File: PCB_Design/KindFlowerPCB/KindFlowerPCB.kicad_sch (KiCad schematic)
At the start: 13 parts, among them J1 LiPo_Connector, J2 FSR_1, J3 Wireless_Charger, J4 FSR_2, J5 FSR_3, J6 FSR_0, J7 NeopixelStrip1, J8 NeopixelStrip2

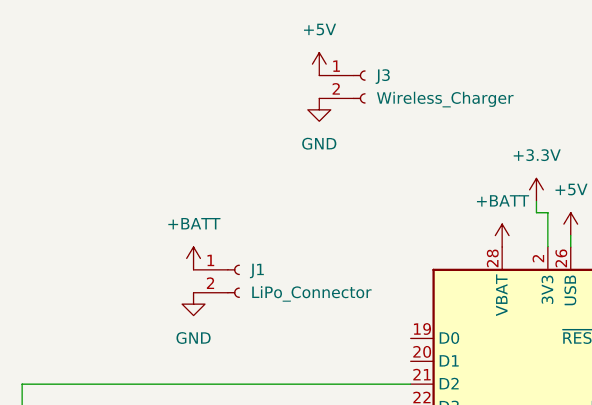
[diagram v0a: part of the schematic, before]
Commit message: PCB file updates
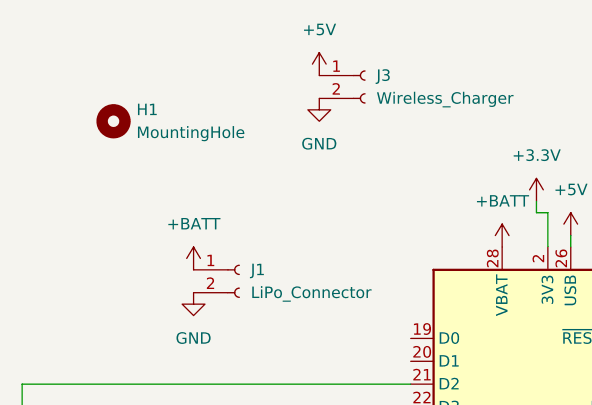
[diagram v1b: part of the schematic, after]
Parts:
- added H1: MountingHole, Images:SmFistBmp, symbol Mechanical:MountingHole
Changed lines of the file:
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@@
+    )
+  )
+  (symbol (lib_id "Mechanical:MountingHole") (at 92.71 39.37 0) (unit 1)
+    (in_bom yes) (on_board yes) (dnp no) (fields_autoplaced)
+    (property "Reference" "H1" (at 95.25 38.1 0)
+      (effects (font (size 1.27 1.27)) (justify left))
+    )
+    (property "Value" "MountingHole" (at 95.25 40.64 0)
+      (effects (font (size 1.27 1.27)) (justify left))
+    )
+    (property "Footprint" "Images:SmFistBmp" (at 92.71 39.37 0)
+      (effects (font (size 1.27 1.27)) hide)
+    )
+    (property "Datasheet" "~" (at 92.71 39.37 0)
+      (effects (font (size 1.27 1.27)) hide)
+    )
+    (instances
+      (project "KindFlowerPCB"
+        (path "/6b2a48b2-d72a-4636-9928-5700417c1281"
+          (reference "H1") (unit 1)
+        )
+      )
     )
   )
